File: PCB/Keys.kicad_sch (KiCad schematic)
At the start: 12 parts, among them U3 DRV5055A3xDBZxQ1, U4 DRV5055A3xDBZxQ1, U5 DRV5055A3xDBZxQ1, U6 DRV5055A3xDBZxQ1

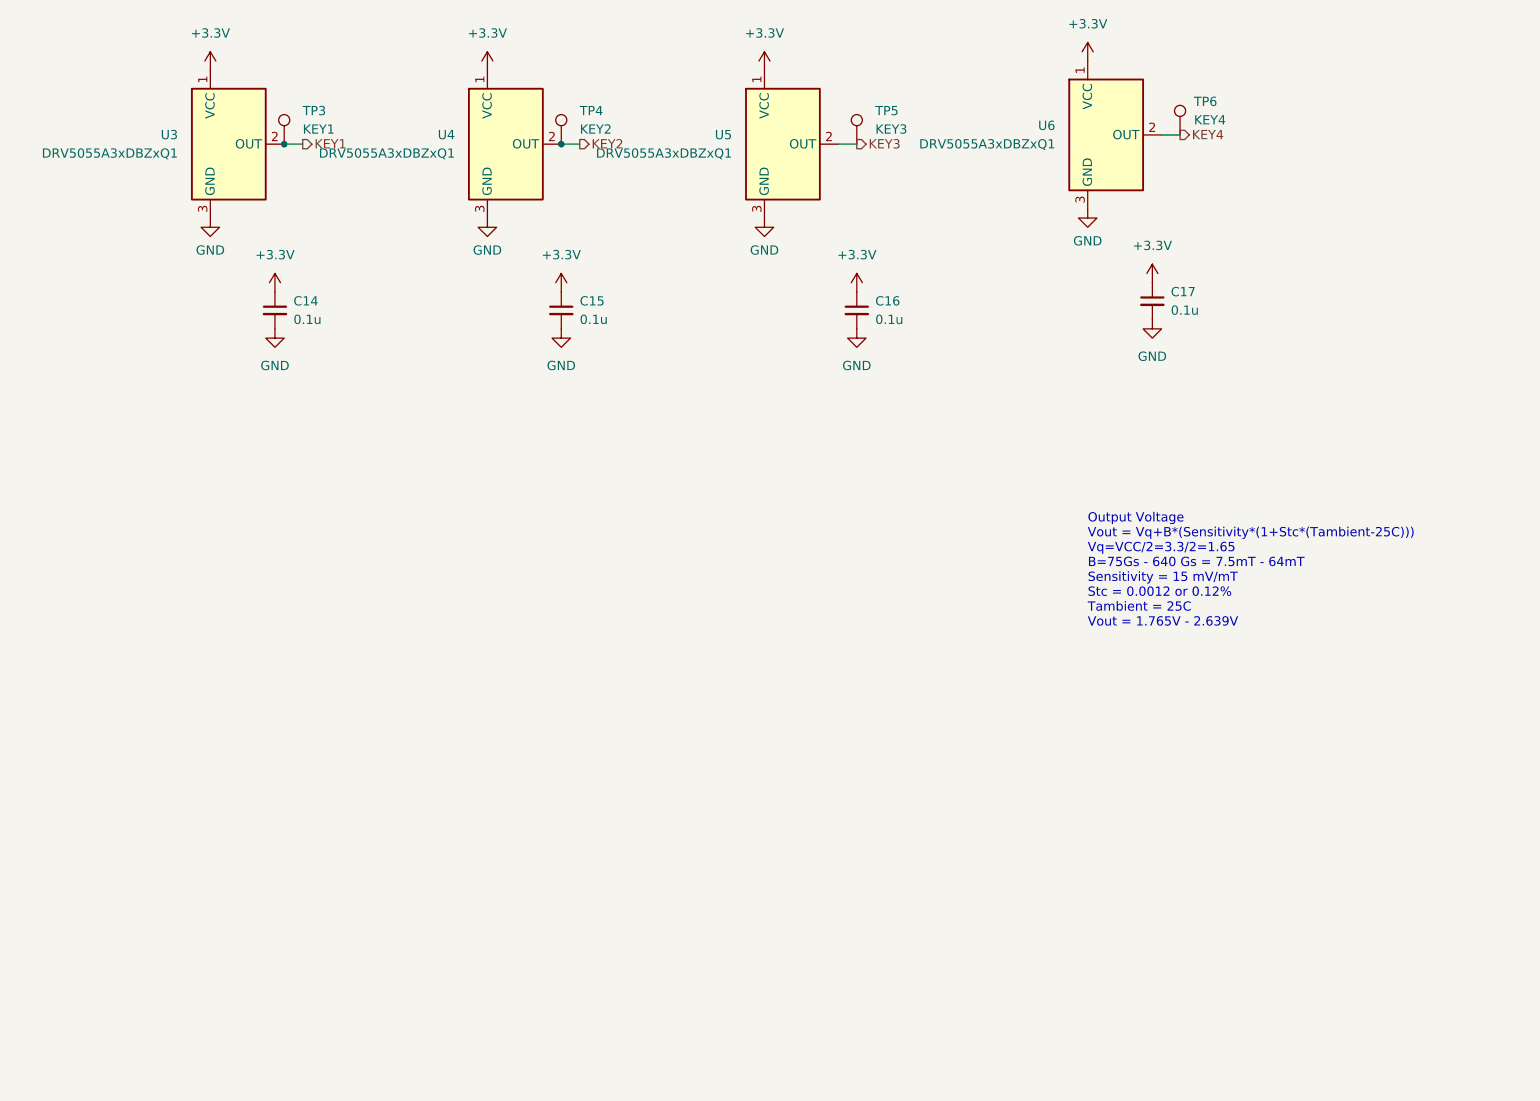
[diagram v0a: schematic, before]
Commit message: analog signal design research
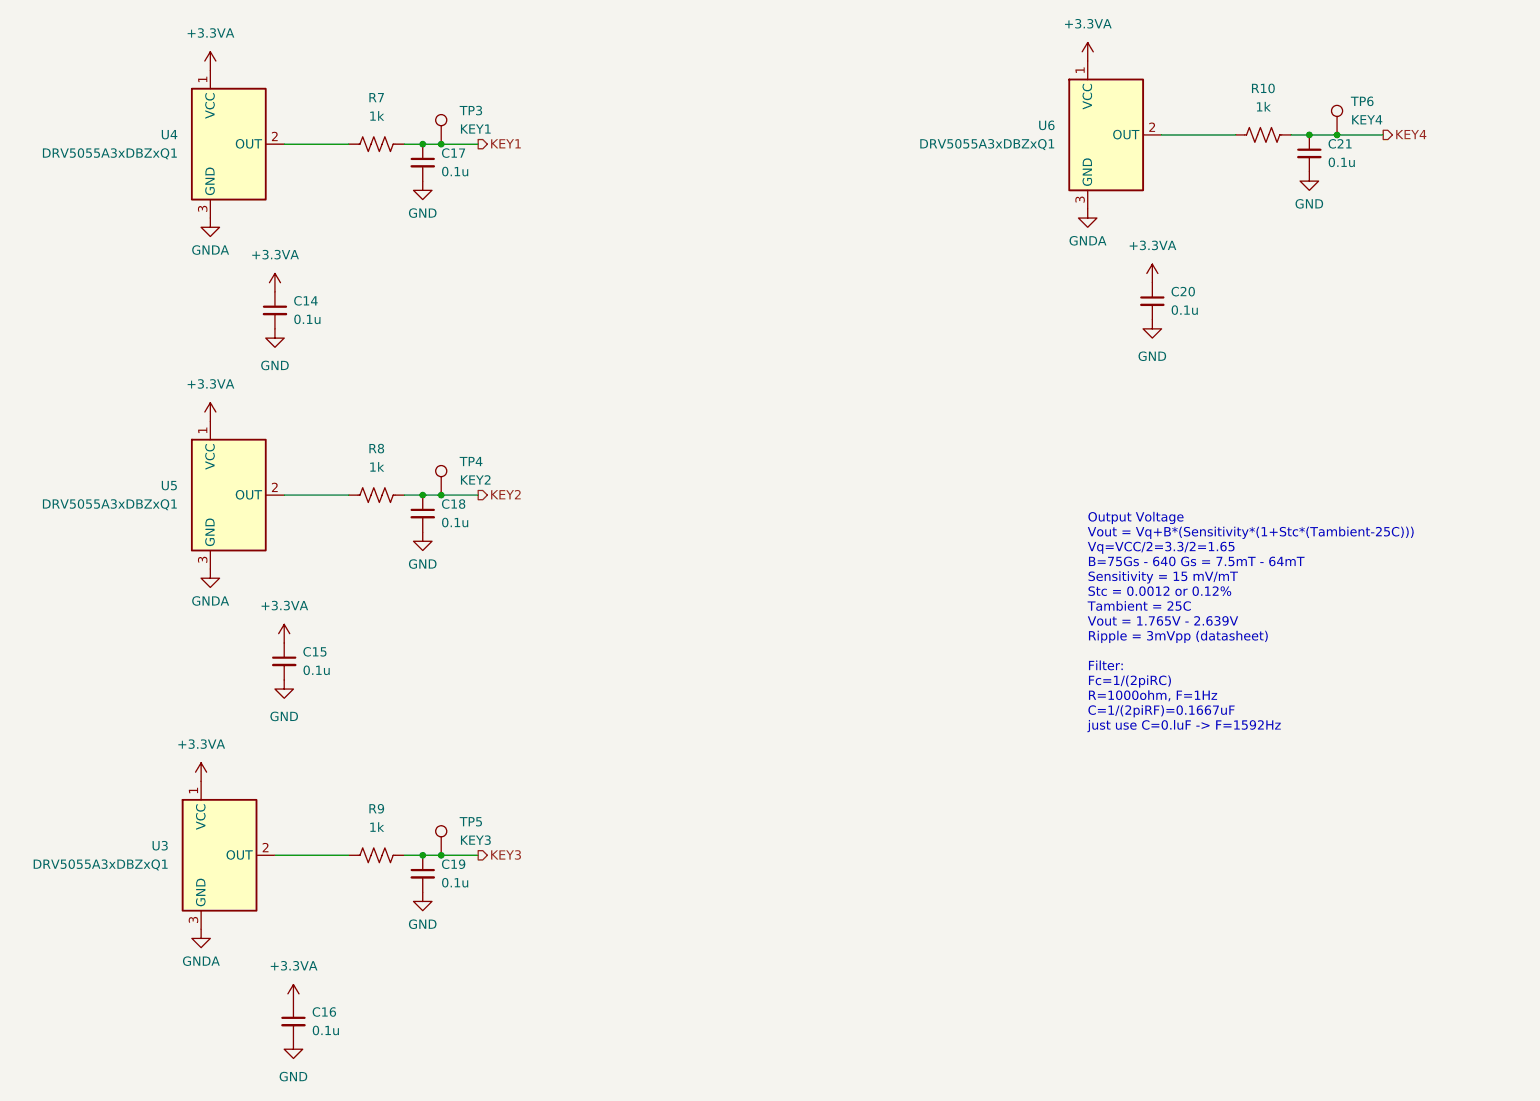
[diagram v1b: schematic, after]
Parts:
- added C17, C18, C19, C21: 0.1u, Capacitor_SMD:C_0603_1608Metric_Pad1.08x0.95mm_HandSolder, symbol Device:C_Small
- added R10, R7, R8, R9: 1k, Resistor_SMD:R_0603_1608Metric_Pad0.98x0.95mm_HandSolder, symbol Device:R_US
- renumbered C17 to C20, U5 to U3, U3 to U4, U4 to U5
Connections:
- net GND: now also C17.2, C18.2, C19.2, C21.2; no longer U3.3 (GND), U4.3 (GND), U5.3 (GND), U6.3 (GND)
- net KEY1: now also C17.1, R7.2; no longer U4.2 (OUT)
- net KEY2: now also C18.1, R8.2; no longer U5.2 (OUT)
- net KEY3: now also C19.1, R9.2; no longer U3.2 (OUT)
- net KEY4: now also C21.1, R10.2; no longer U6.2 (OUT)
- net +3.3V renamed +3.3VA
- new net: R7.1, U4.2 (OUT)
- new net: R9.1, U3.2 (OUT)
- new net: R8.1, U5.2 (OUT)
- new net: R10.1, U6.2 (OUT)
- new net GNDA: U3.3 (GND), U4.3 (GND), U5.3 (GND), U6.3 (GND)
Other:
- note added: "Output Voltage Vout = Vq+B*(Sensitivity*(1+Stc*(Tambient-25C))) Vq=VCC/2=3.3/2=1.65 B=75Gs - 640 Gs = 7.5mT - 64mT Sensitivity = 15 mV/mT Stc = 0.0012 or 0.12% Tambient = 25C Vout = 1.765V - 2.639V Ripple = 3mVpp (datasheet) Filter: Fc=1/(2piRC) R=1000ohm, F=1Hz C=1/(2piRF)=0.1667uF just use C=0.luF -> F=1592Hz"
- note removed: "Output Voltage Vout = Vq+B*(Sensitivity*(1+Stc*(Tambient-25C))) Vq=VCC/2=3.3/2=1.65 B=75Gs - 640 Gs = 7.5mT - 64mT Sensitivity = 15 mV/mT Stc = 0.0012 or 0.12% Tambient = 25C Vout = 1.765V - 2.639V"
- moved on the sheet: C15, C16, TP3, TP4, TP5, TP6, U3, U5
